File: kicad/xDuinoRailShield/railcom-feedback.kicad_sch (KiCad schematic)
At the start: 8 parts, among them Q401 S8050, Q402 S8550, Q403 S8550, Q404 S8050

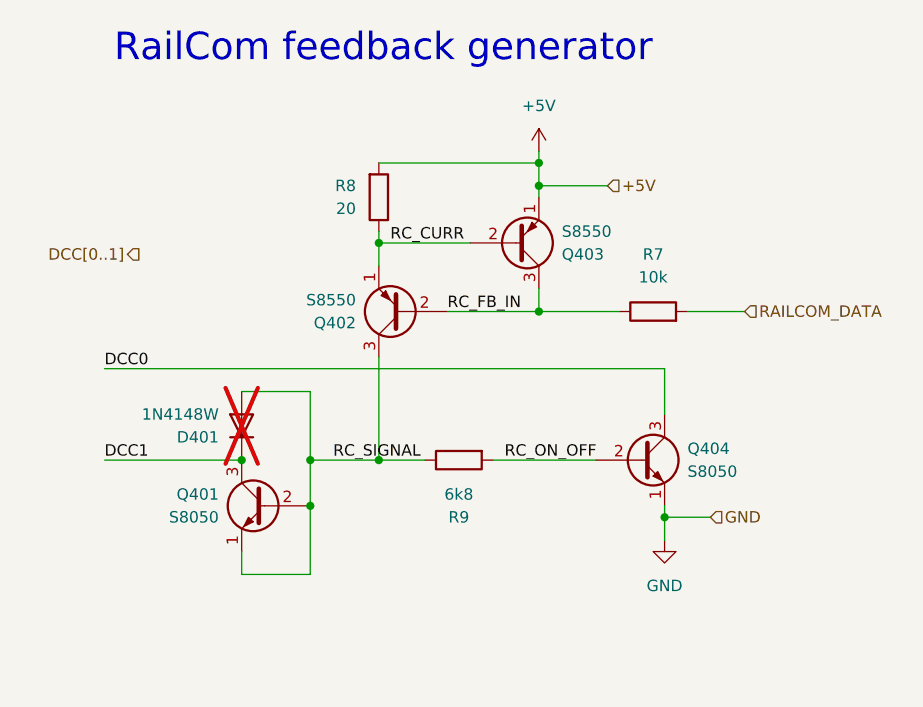
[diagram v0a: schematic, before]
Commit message: Final version
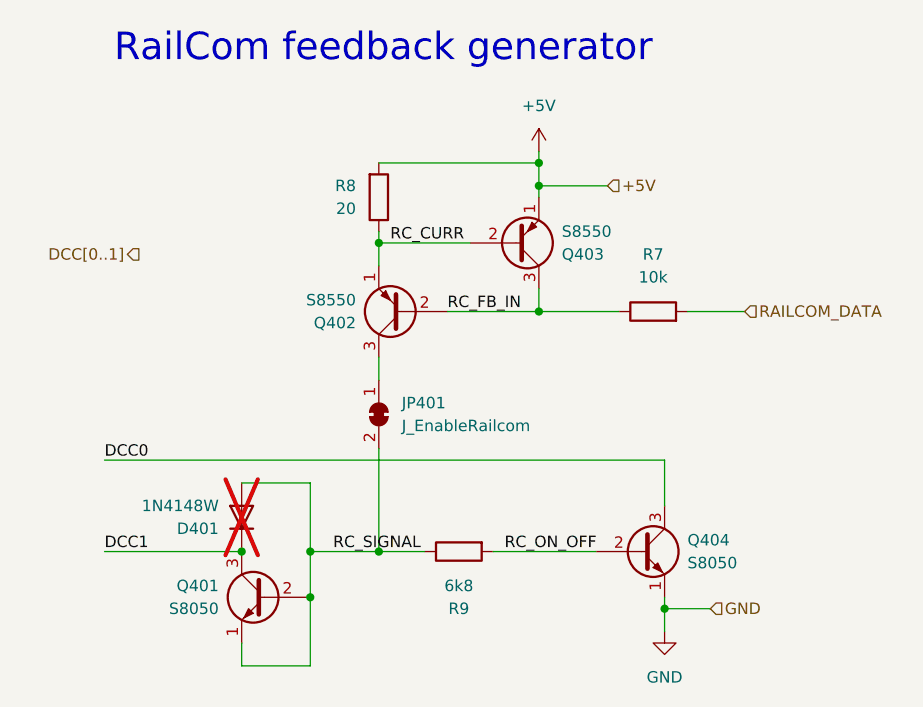
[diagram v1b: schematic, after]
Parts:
- added JP401: J_EnableRailcom, Jumper:SolderJumper-2_P1.3mm_Bridged_RoundedPad1.0x1.5mm, symbol Jumper:SolderJumper_2_Bridged
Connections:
- net RC_SIGNAL: now also JP401.2 (B); no longer Q402.3 (C)
- new net: JP401.1 (A), Q402.3 (C)
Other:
- moved on the sheet: D401, Q401, Q404, R9

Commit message: Refactoring & Sound
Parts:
- R7, R8, R9: footprint Resistor_SMD:R_0805_2012Metric_Pad1.20x1.40mm_HandSolder -> Resistor_SMD:R_0402_1005Metric_Pad0.72x0.64mm_HandSolder
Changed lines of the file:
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@@
 			)
 		)
-		(property "Footprint" "Resistor_SMD:R_0805_2012Metric_Pad1.20x1.40mm_HandSolder"
+		(property "Footprint" "Resistor_SMD:R_0402_1005Metric_Pad0.72x0.64mm_HandSolder"
 			(at 93.98 58.928 90)
 			(effects
@@
 			)
 		)
-		(property "Footprint" "Resistor_SMD:R_0805_2012Metric_Pad1.20x1.40mm_HandSolder"
+		(property "Footprint" "Resistor_SMD:R_0402_1005Metric_Pad0.72x0.64mm_HandSolder"
 			(at 61.722 44.45 90)
 			(effects
@@
 			)
 		)
-		(property "Footprint" "Resistor_SMD:R_0805_2012Metric_Pad1.20x1.40mm_HandSolder"
+		(property "Footprint" "Resistor_SMD:R_0402_1005Metric_Pad0.72x0.64mm_HandSolder"
 			(at 72.39 82.042 90)
 			(effects
